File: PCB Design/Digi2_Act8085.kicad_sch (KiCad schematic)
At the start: 20 parts, among them U1 8085A, U2 Barrel_Jack, U3 L7805, Y1 3MHz

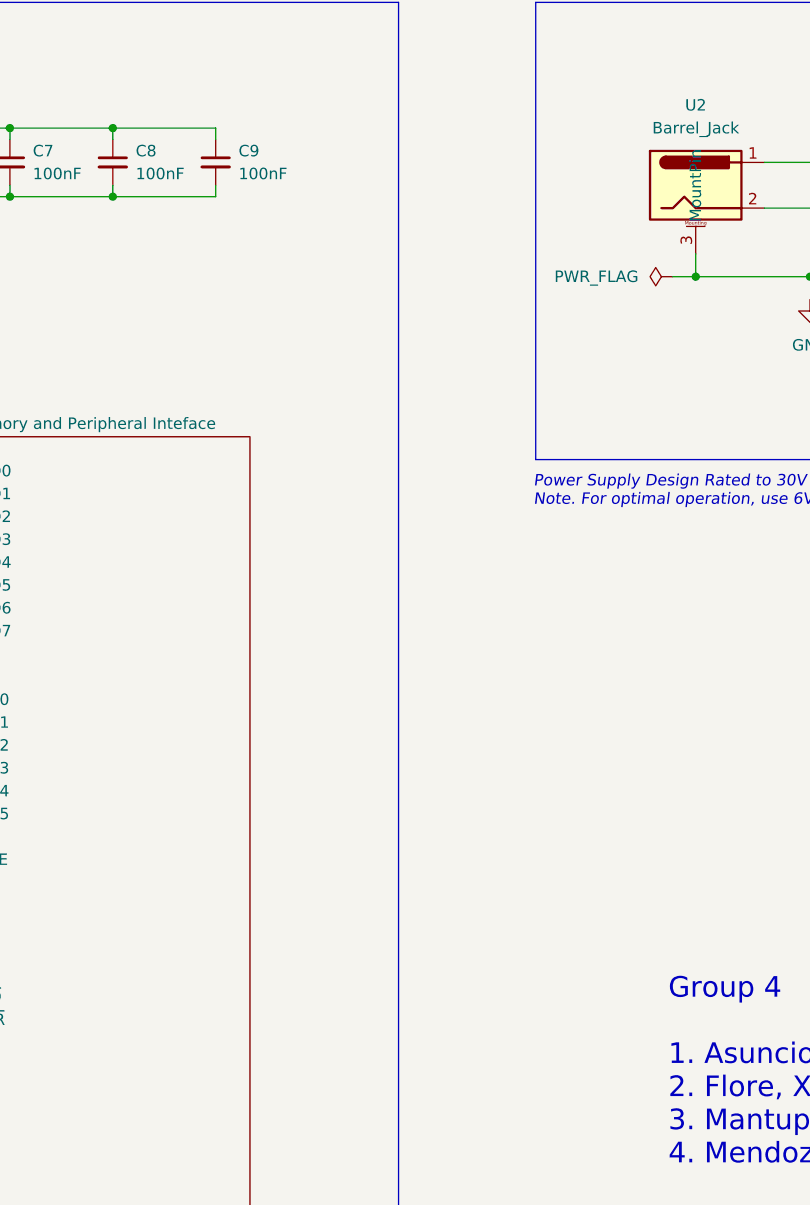
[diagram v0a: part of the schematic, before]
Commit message: Add ground
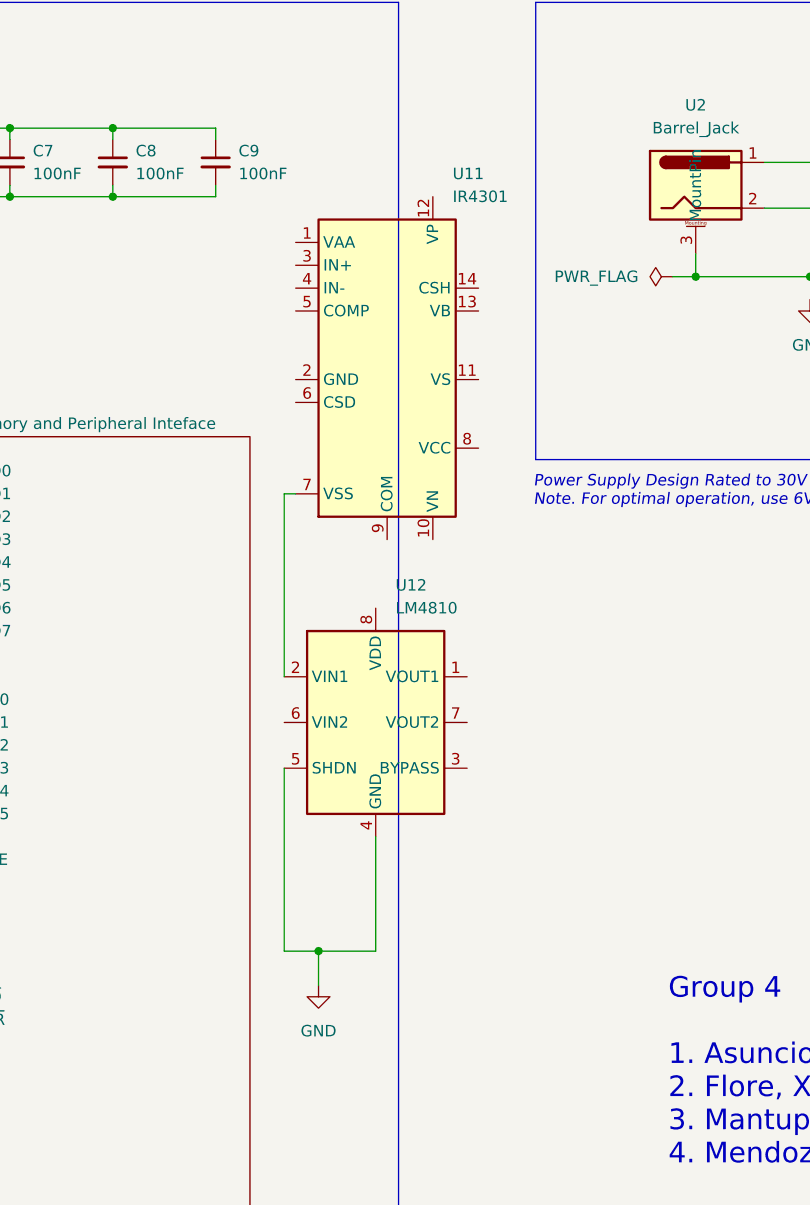
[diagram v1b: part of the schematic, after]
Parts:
- added U11: IR4301, Package_DFN_QFN:Infineon_PQFN-22-15-4EP_6x5mm_P0.65mm, symbol Amplifier_Audio:IR4301
- added U12: LM4810, Package_SO:TSSOP-8_3x3mm_P0.65mm, symbol Amplifier_Audio:LM4810
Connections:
- net GND: now also U12.4 (GND), U12.5 (SHDN)
- new net: U11.7 (VSS), U12.2 (VIN1)
- new net: U11.15 (COM), U11.9 (COM)

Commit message: Remove Not needed
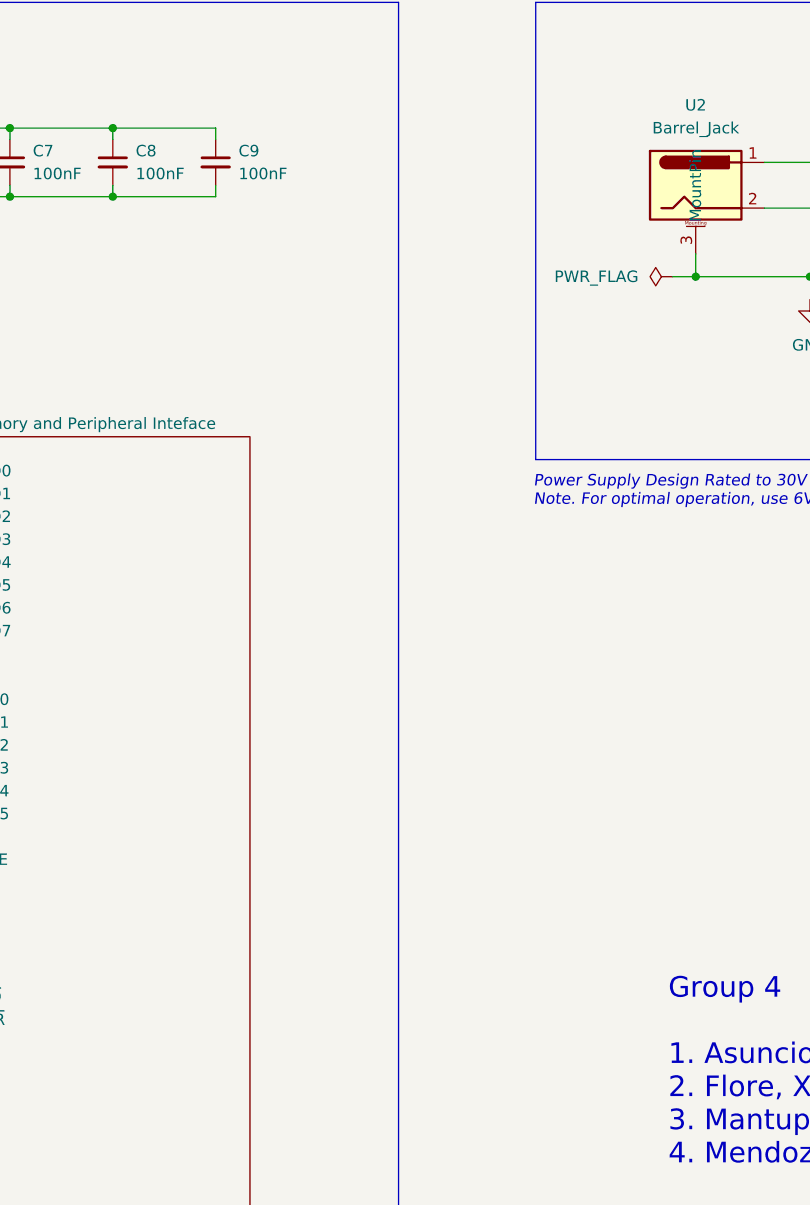
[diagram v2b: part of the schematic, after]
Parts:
- removed U11: IR4301, Package_DFN_QFN:Infineon_PQFN-22-15-4EP_6x5mm_P0.65mm, symbol Amplifier_Audio:IR4301
- removed U12: LM4810, Package_SO:TSSOP-8_3x3mm_P0.65mm, symbol Amplifier_Audio:LM4810

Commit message: Updated PCB and Footprint
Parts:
- C1, C11: footprint Capacitor_THT:CP_Radial_D8.0mm_P3.50mm -> Capacitor_THT:CP_Radial_D5.0mm_P2.50mm
- C10: footprint Capacitor_THT:CP_Radial_D8.0mm_P3.50mm -> Capacitor_THT:CP_Radial_D4.0mm_P2.00mm
- C12: footprint Capacitor_THT:CP_Radial_D8.0mm_P3.50mm -> Capacitor_THT:C_Disc_D4.3mm_W1.9mm_P5.00mm
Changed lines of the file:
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@@
 			)
 		)
-		(property "Footprint" "Capacitor_THT:CP_Radial_D8.0mm_P3.50mm"
+		(property "Footprint" "Capacitor_THT:C_Disc_D4.3mm_W1.9mm_P5.00mm"
 			(at 43.18 127 0)
 			(effects
@@
 			)
 		)
-		(property "Footprint" "Capacitor_THT:CP_Radial_D8.0mm_P3.50mm"
+		(property "Footprint" "Capacitor_THT:CP_Radial_D5.0mm_P2.50mm"
 			(at 36.83 44.45 0)
 			(effects
@@
 			)
 		)
-		(property "Footprint" "Capacitor_THT:CP_Radial_D8.0mm_P3.50mm"
+		(property "Footprint" "Capacitor_THT:CP_Radial_D5.0mm_P2.50mm"
 			(at 252.4252 54.61 0)
 			(effects
@@
 			)
 		)
-		(property "Footprint" "Capacitor_THT:CP_Radial_D8.0mm_P3.50mm"
+		(property "Footprint" "Capacitor_THT:CP_Radial_D4.0mm_P2.00mm"
 			(at 223.2152 54.61 0)
 			(effects
